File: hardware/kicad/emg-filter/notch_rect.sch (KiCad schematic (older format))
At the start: 24 parts, among them U1 LM4565, U2 LM4565

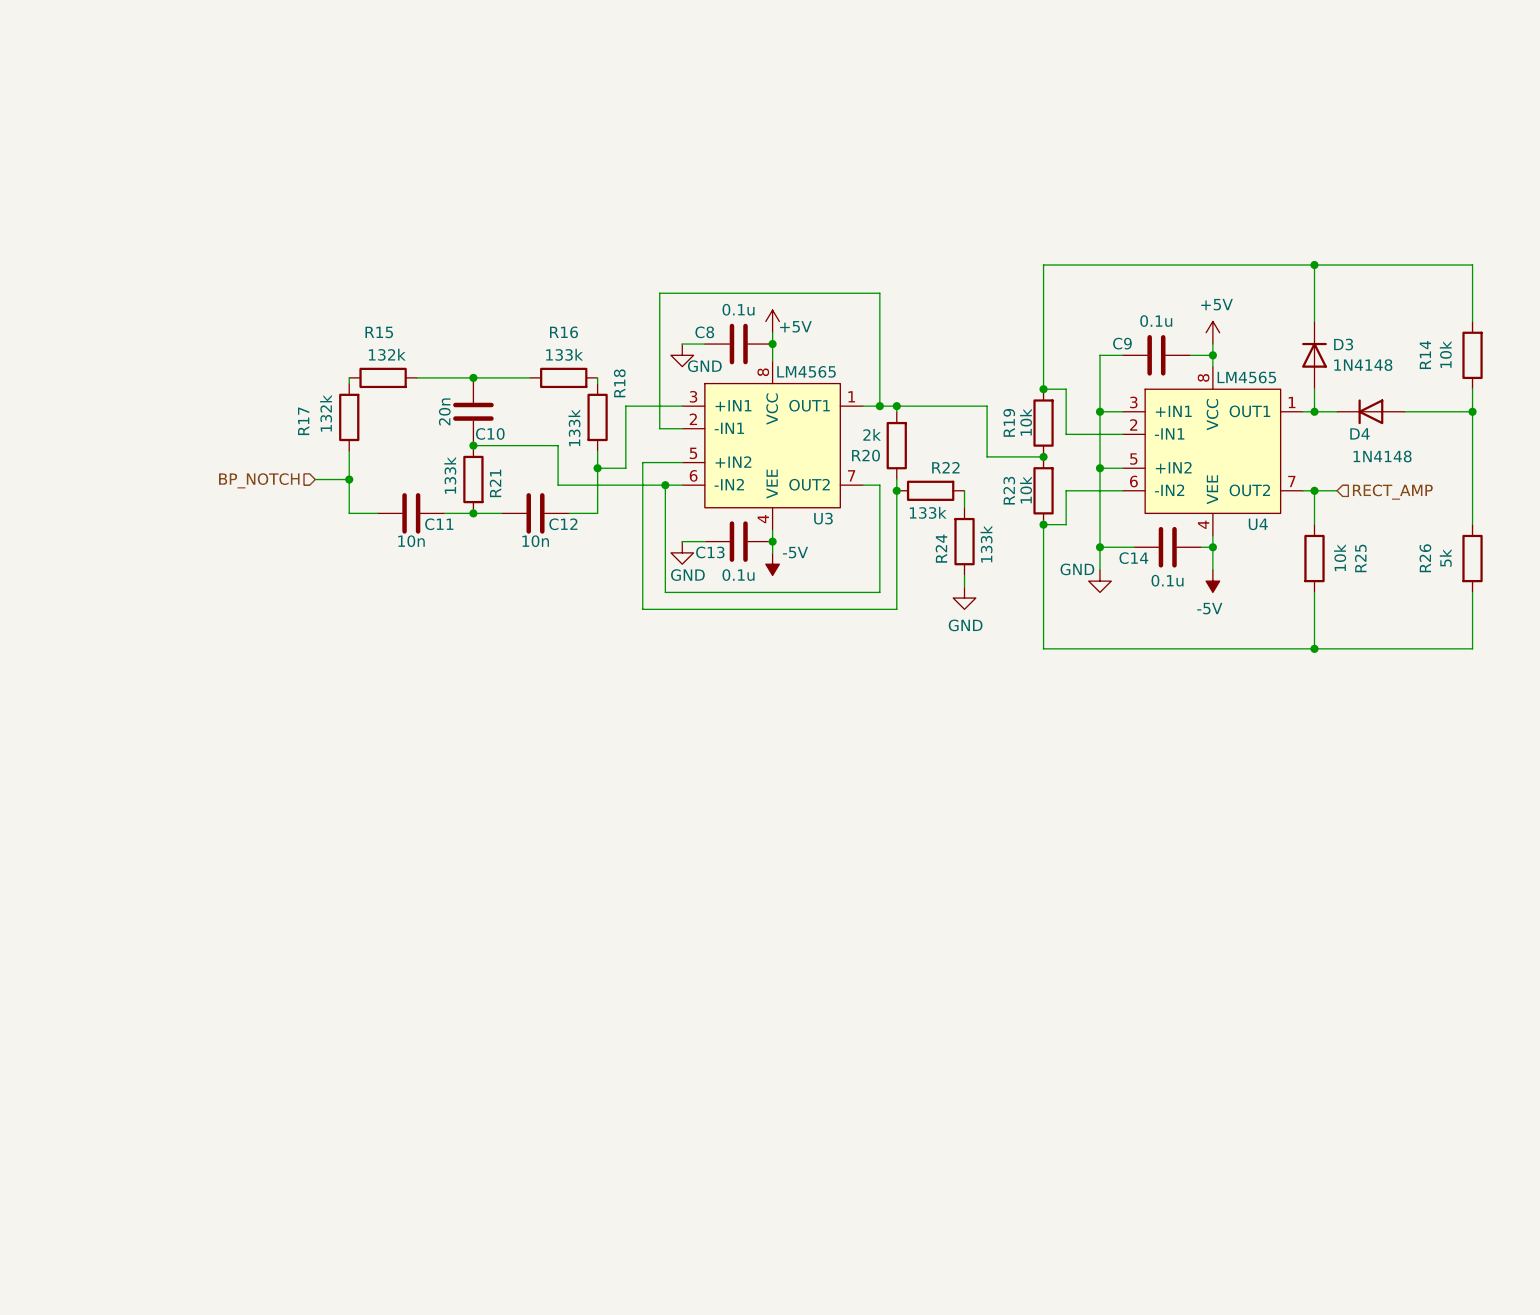
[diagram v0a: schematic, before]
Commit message: update
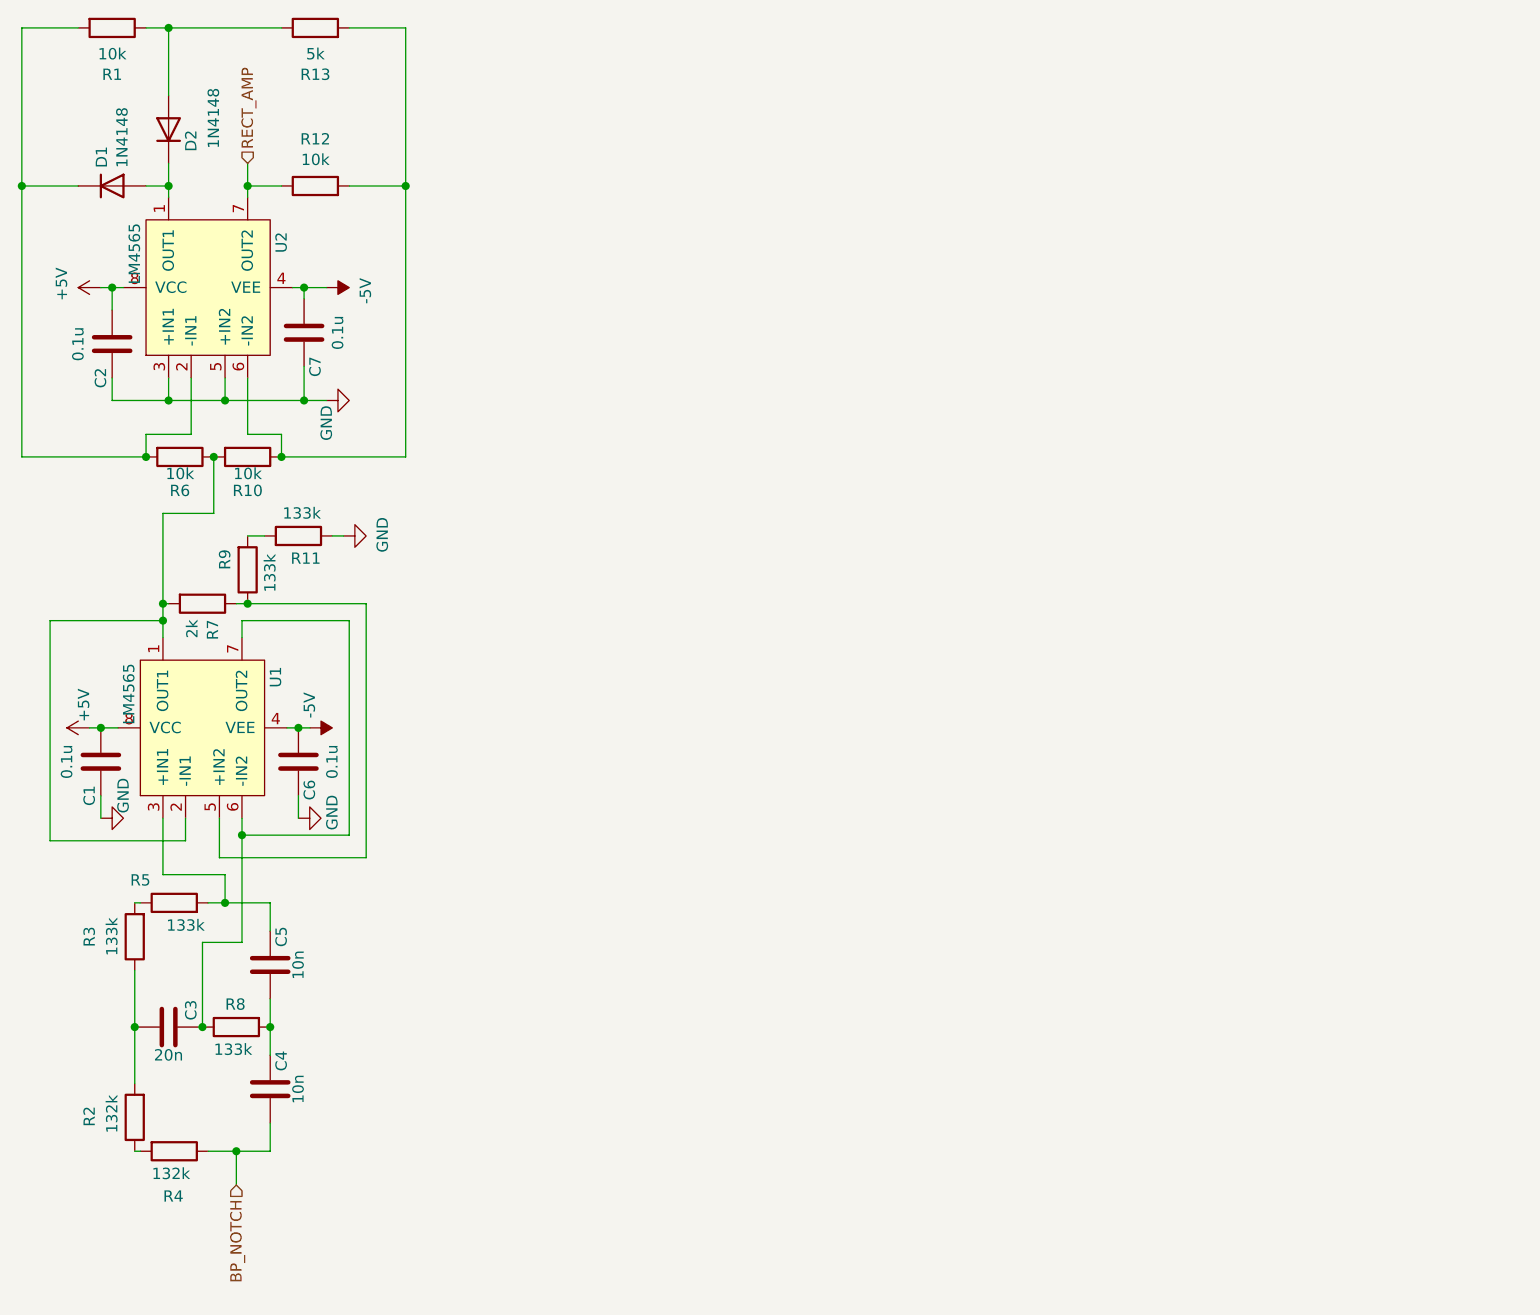
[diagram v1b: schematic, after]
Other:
- moved on the sheet: C1, C2, C3, C4, C5, C6, C7, D1, D2, R1, R10, R11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

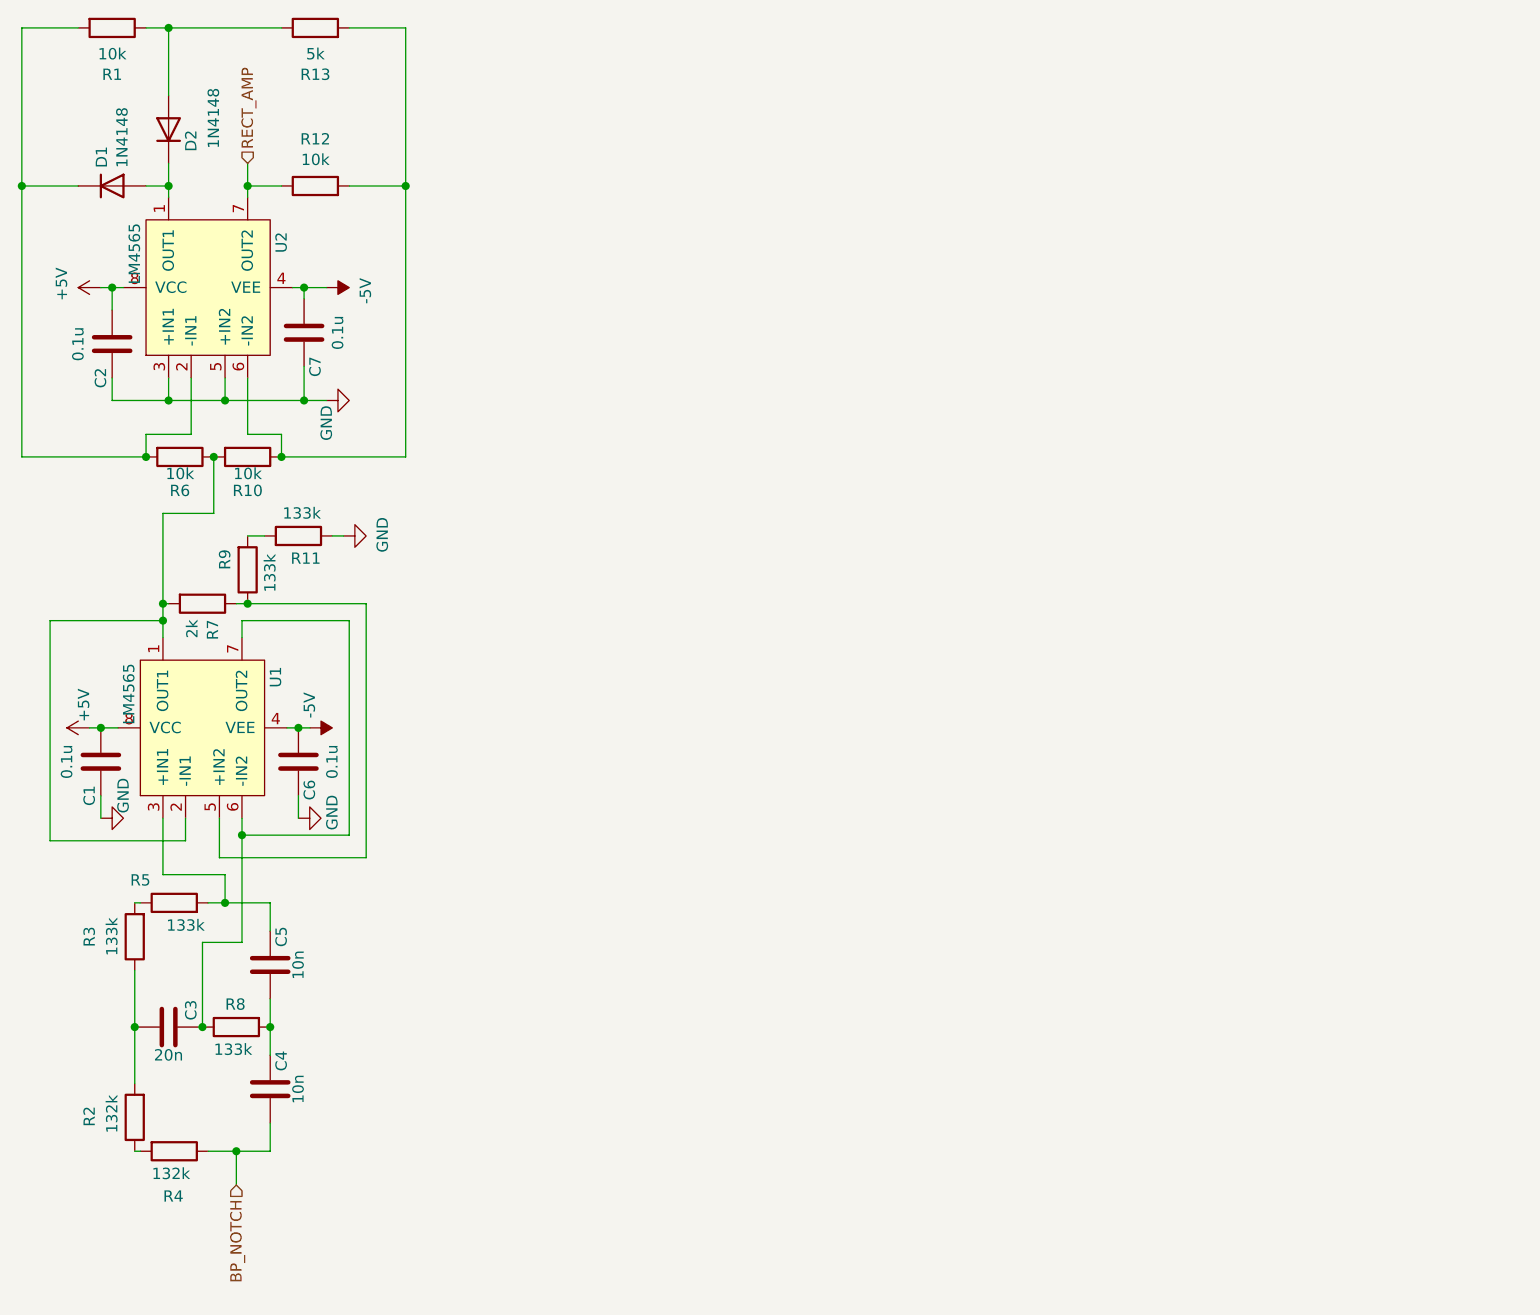
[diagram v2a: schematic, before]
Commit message: update
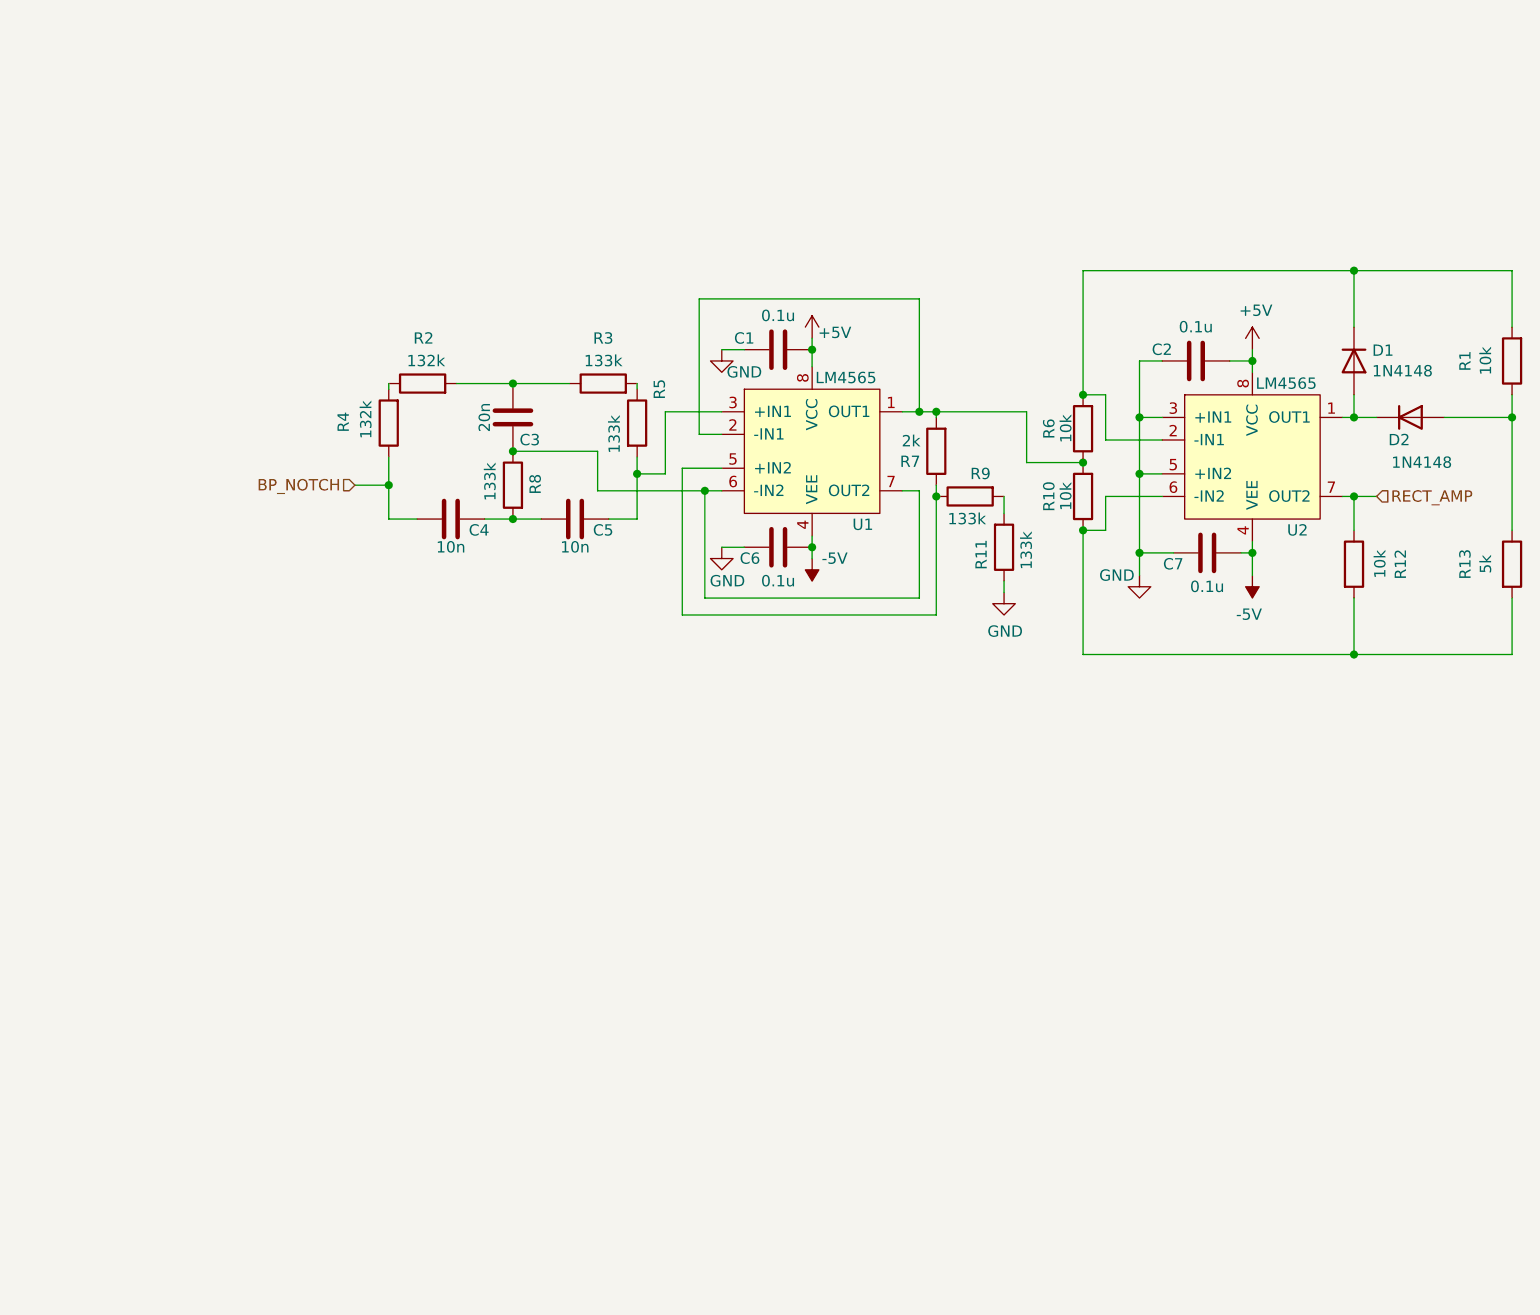
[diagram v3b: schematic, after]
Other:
- moved on the sheet: C1, C2, C3, C4, C5, C6, C7, D1, D2, R1, R10, R11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
